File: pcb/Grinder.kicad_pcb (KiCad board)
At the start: 2 copper layers, 43.2 x 57.1 mm, 8 parts

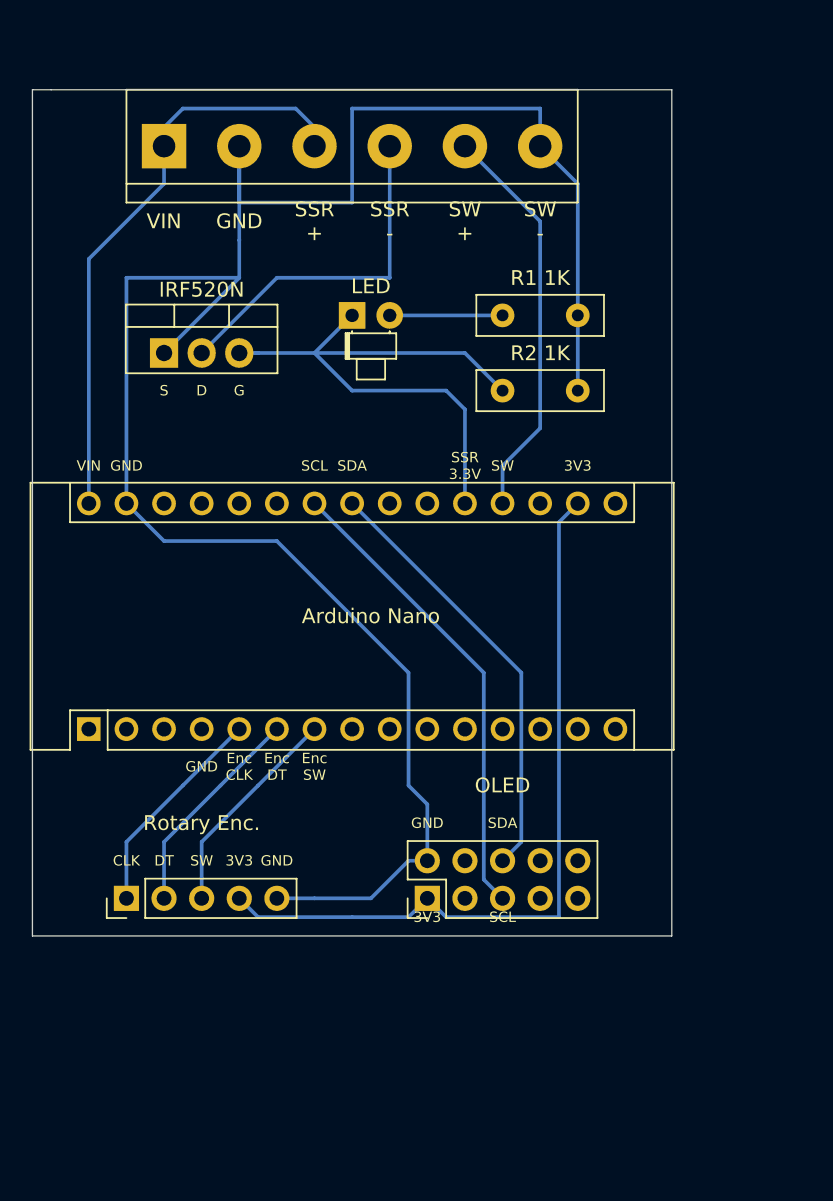
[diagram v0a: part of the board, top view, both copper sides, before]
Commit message: WIP for new PCB
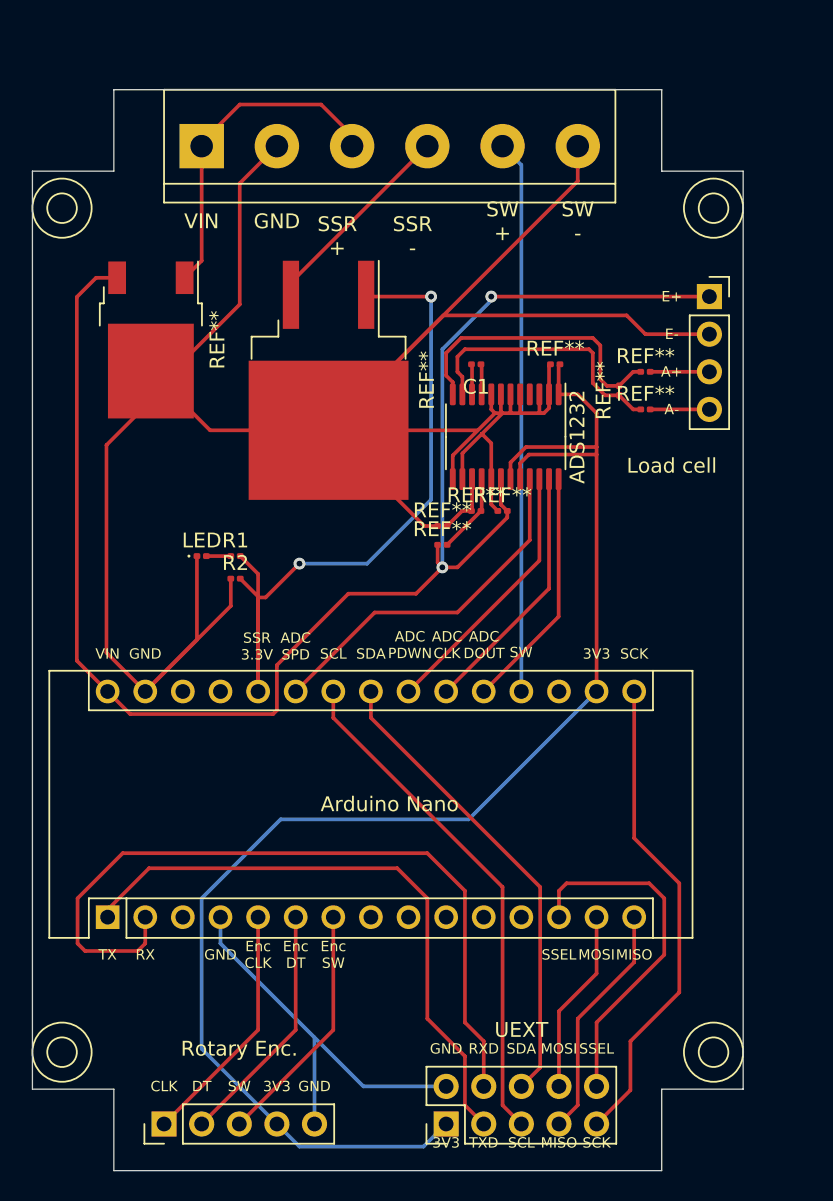
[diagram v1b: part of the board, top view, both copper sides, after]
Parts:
- removed IRF520N: TO-220-3_Vertical, Package_TO_SOT_THT:TO-220-3_Vertical
- removed the LED at (148.6, 59.7)
- removed R1 1K: R_Box_L8.4mm_W2.5mm_P5.08mm, Resistor_THT:R_Box_L8.4mm_W2.5mm_P5.08mm
- removed R2 1K: R_Box_L8.4mm_W2.5mm_P5.08mm, Resistor_THT:R_Box_L8.4mm_W2.5mm_P5.08mm
- added ADS1232: TSSOP-24_4.4x7.8mm_P0.65mm, Package_SO:TSSOP-24_4.4x7.8mm_P0.65mm, F.Cu at (159.0, 67.9)
- added C1: C_0201_0603Metric, Capacitor_SMD:C_0201_0603Metric, F.Cu at (157.0, 63.0)
- added LED: LED_0201_0603Metric, LED_SMD:LED_0201_0603Metric, F.Cu at (138.4, 75.9)
- added Load cell: PinSocket_1x04_P2.54mm_Vertical, Connector_PinSocket_2.54mm:PinSocket_1x04_P2.54mm_Vertical, F.Cu at (172.7, 58.4)
- added R1: R_0201_0603Metric, Resistor_SMD:R_0201_0603Metric, F.Cu at (140.7, 75.9)
- added R2: R_0201_0603Metric, Resistor_SMD:R_0201_0603Metric, F.Cu at (140.7, 77.5)
- added REF**: C_0201_0603Metric, Capacitor_SMD:C_0201_0603Metric, F.Cu at (158.8, 72.9)
- added REF**: R_0201_0603Metric, Resistor_SMD:R_0201_0603Metric, F.Cu at (168.4, 66.0)
- added REF**: R_0201_0603Metric, Resistor_SMD:R_0201_0603Metric, F.Cu at (168.4, 63.5)
- added REF**: R_0201_0603Metric, Resistor_SMD:R_0201_0603Metric, F.Cu at (154.7, 75.2)
- added REF**: R_0201_0603Metric, Resistor_SMD:R_0201_0603Metric, F.Cu at (154.7, 73.9)
- added REF**: C_0201_0603Metric, Capacitor_SMD:C_0201_0603Metric, F.Cu at (157.0, 72.9)
- added REF**: Battery_CR1225, Battery:Battery_CR1225, F.Cu at (142.0, 75.9)
- added REF**: TO-263-2, Package_TO_SOT_SMD:TO-263-2, F.Cu at (147.0, 64.1)
- added REF**: TO-252-2, Package_TO_SOT_SMD:TO-252-2, F.Cu at (135.0, 61.4)
- added REF**: C_0201_0603Metric, Capacitor_SMD:C_0201_0603Metric, F.Cu at (162.3, 63.0)
- added REF**: C_0201_0603Metric, Capacitor_SMD:C_0201_0603Metric, F.Cu at (166.6, 64.8)
- moved Rotary Enc. 15.5 mm to (135.9, 114.3)
- moved UEXT 15.3 mm to (154.9, 114.3)
- moved Arduino Nano 12.8 mm to (132.1, 100.3)
- moved REF** 2.54 mm to (138.4, 48.3)
- renumbered OLED to UEXT
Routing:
- net (no net): track 434.8 -> 972.4 mm, vias 0 -> 4
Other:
- board size 43.2 x 57.1 mm -> 48 x 73 mm
- net class 5V added: clearance 0.2, trace_width 0.25, via_dia 0.8, via_drill 0.4
- net class 9V added: clearance 0.2, trace_width 0.25, via_dia 0.8, via_drill 0.4
- board text added: "A+"
- board text added: "A-"
- board text added: "ADC CLK"
- board text added: "ADC DOUT"
- board text added: "ADC PDWN"
- board text added: "ADC SPD"
- board text added: "E+"
- board text added: "E-"
- board text added: "MISO"
- board text added: "MOSI"
- board text added: "RX"
- board text added: "RXD"
- board text added: "SCK"
- board text added: "SSEL"
- board text added: "TX"
- board text added: "TXD"
- board text removed: "D"
- board text removed: "G"
- board text removed: "S"
